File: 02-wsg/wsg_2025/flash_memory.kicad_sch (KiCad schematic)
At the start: 2 parts, among them IC1 W25N04KVZEIR

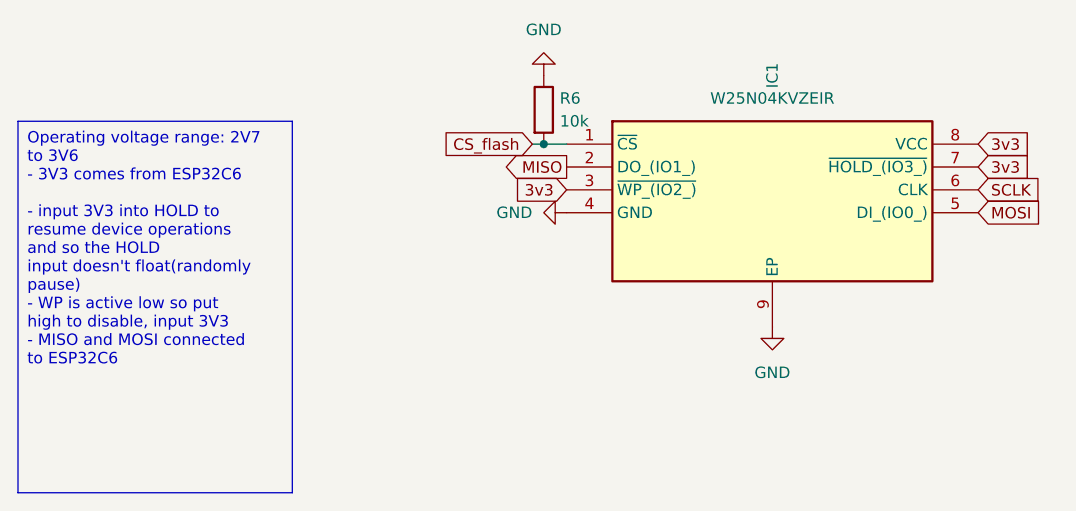
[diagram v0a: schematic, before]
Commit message: new wsg schem - not complete
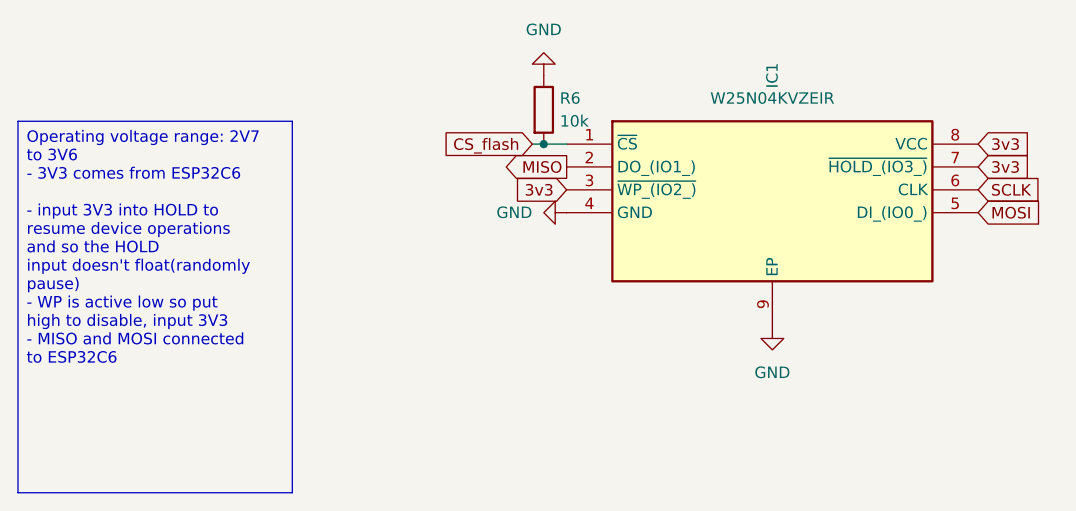
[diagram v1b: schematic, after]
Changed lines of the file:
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@@
 (kicad_sch
-	(version 20231120)
+	(version 20250114)
 	(generator "eeschema")
-	(generator_version "8.0")
+	(generator_version "9.0")
 	(paper "A4")
+	(text_box "Operating voltage range: 2V7 to 3V6\n- 3V3 comes from ESP32C6\n\n- input 3V3 into HOLD to resume device operations and so the HOLD\ninput doesn't float(randomly pause)\n- WP is active low so put high to disable, input 3V3\n- MISO and MOSI connected to ESP32C6"
+		(exclude_from_sim no)
+		(at 52.07 81.28 0)
+		(size 30.48 41.275)
+		(margins 0.9525 0.9525 0.9525 0.9525)
+		(stroke
+			(width 0)
+			(type default)
+		)
+		(fill
+			(type none)
+		)
+		(effects
+			(font
+				(size 1.27 1.27)
+			)
+			(justify left top)
+		)
+	)
 	(junction
 		(at 110.49 83.82)
@@
 		)
 	)
-	(text_box "Operating voltage range: 2V7 to 3V6\n- 3V3 comes from ESP32C6\n\n- input 3V3 into HOLD to resume device operations and so the HOLD\ninput doesn't float(randomly pause)\n- WP is active low so put high to disable, input 3V3\n- MISO and MOSI connected to ESP32C6"
-		(exclude_from_sim no)
-		(at 52.07 81.28 0)
-		(size 30.48 41.275)
-		(stroke
-			(width 0)
-			(type default)
-		)
-		(fill
-			(type none)
-		)
-		(effects
-			(font
-				(size 1.27 1.27)
-			)
-			(justify left top)
-		)
-	)
